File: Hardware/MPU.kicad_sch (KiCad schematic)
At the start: 18 parts, among them J6 USB_C_Receptacle_USB2.0_16P, U14 AP2112K-3.3, U2 STM32H723VGTx

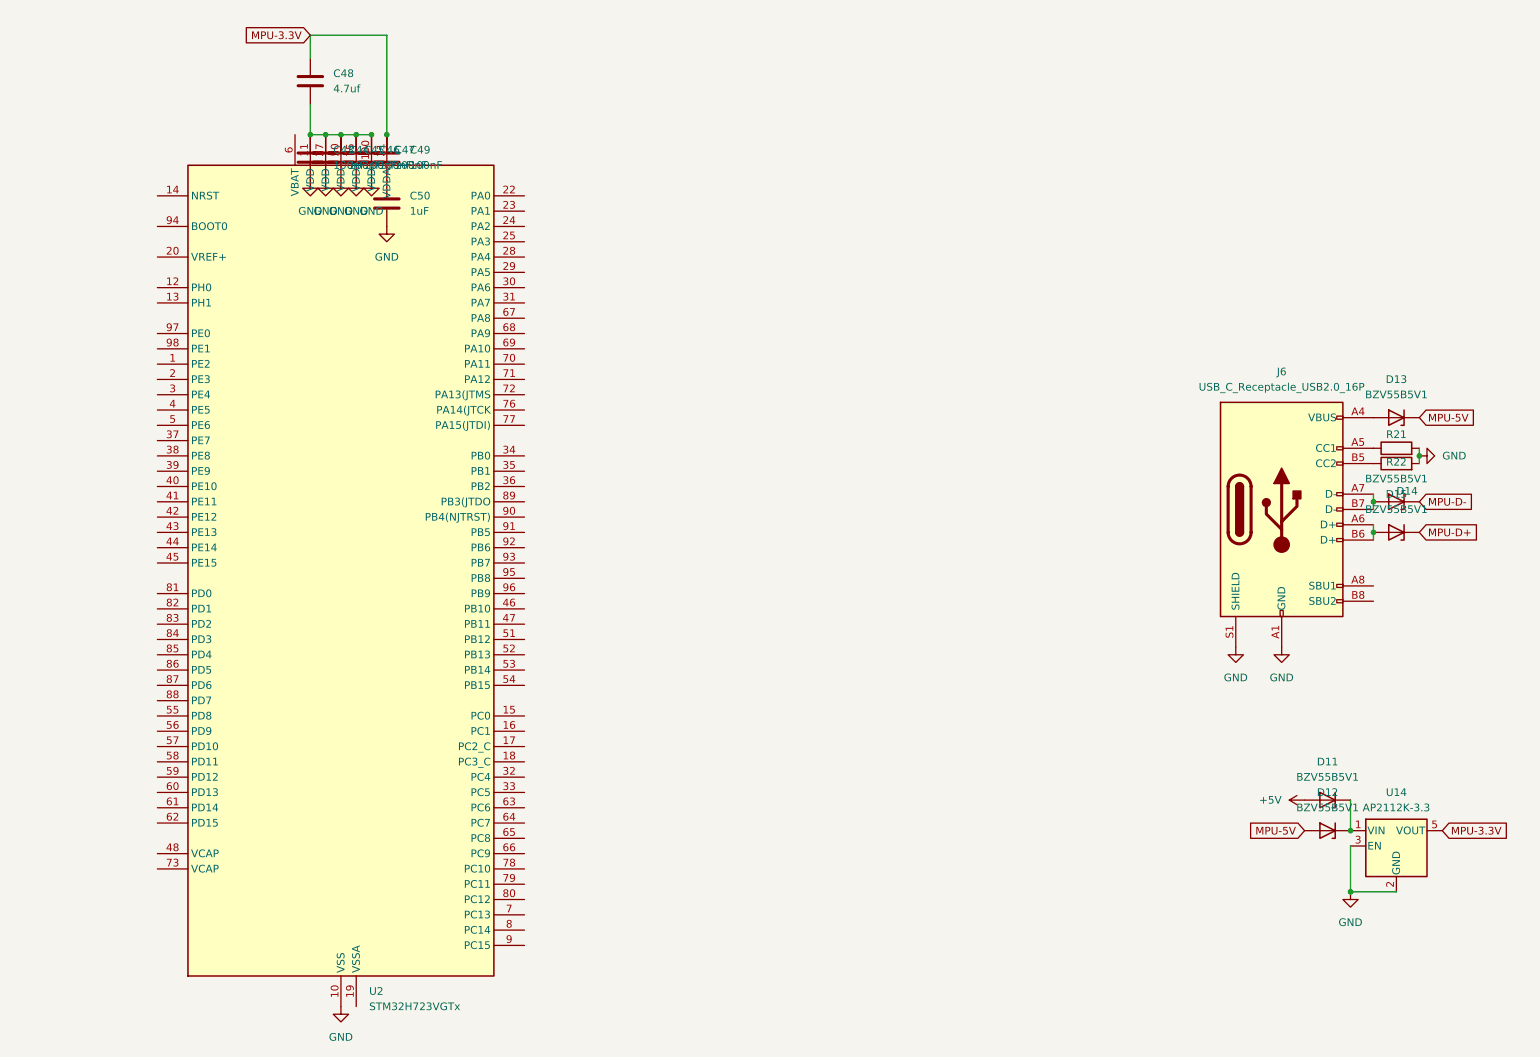
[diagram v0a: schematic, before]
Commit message: 19-feb update
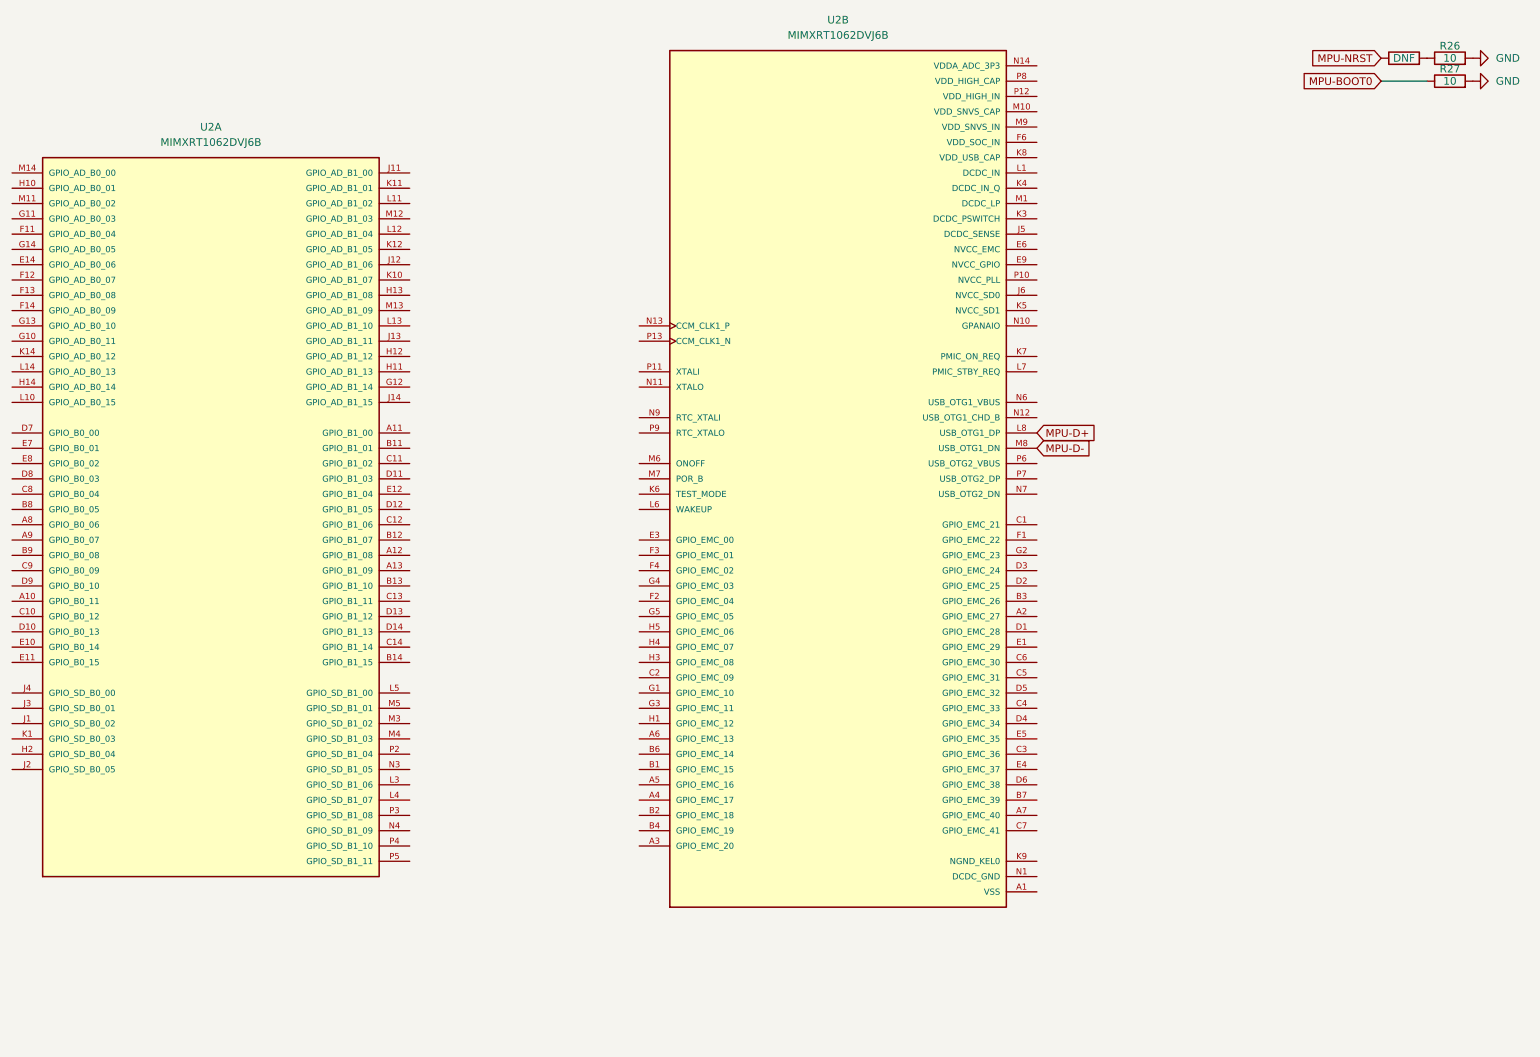
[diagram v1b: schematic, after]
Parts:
- removed C43, C44, C45, C46, C47, C49: 100nF, Capacitor_SMD:C_0201_0603Metric, symbol Device:C
- removed C48: 4.7uf, Capacitor_SMD:C_0603_1608Metric, symbol Device:C
- removed C50: 1uF, Capacitor_SMD:C_0201_0603Metric, symbol Device:C
- removed D11, D12, D13, D14, D15: BZV55B5V1, Diode_SMD:D_MiniMELF, symbol Diode:BZV55B5V1
- removed J6: USB_C_Receptacle_USB2.0_16P, Connector_USB:USB_C_Receptacle_G-Switch_GT-USB-7010ASV, symbol Connector:USB_C_Receptacle_USB2.0_16P
- removed R21, R22: R, Resistor_SMD:R_01005_0402Metric_Pad0.57x0.30mm_HandSolder, symbol Device:R
- removed U14: AP2112K-3.3, Package_TO_SOT_SMD:SOT-23-5, symbol Regulator_Linear:AP2112K-3.3
- removed U2: STM32H723VGTx, Package_QFP:LQFP-100_14x14mm_P0.5mm, symbol MCU_ST_STM32H7:STM32H723VGTx
- added R25: DNF, Resistor_SMD:R_0603_1608Metric, symbol Device:R
- added R26, R27: 10, Resistor_SMD:R_0201_0603Metric_Pad0.64x0.40mm_HandSolder, symbol Device:R
- added U2: MIMXRT1062DVJ6B, MIMXRT1062DVJ6B:BGA196C80P14X14_1200X1200X152N, symbol MIMXRT1062DVJ6B:MIMXRT1062DVJ6B
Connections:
- net GND: now also R26.2, R27.2
- net MPU-D+: now also U2.L8 (USB_OTG1_DP)
- net MPU-D-: now also U2.M8 (USB_OTG1_DN)
- new net: R25.2, R26.1
- new net DCDC_GND: U2.N1 (DCDC_GND), U2.N2 (DCDC_GND)
- new net DCDC_IN: U2.L1 (DCDC_IN), U2.L2 (DCDC_IN)
- new net DCDC_LP: U2.M1 (DCDC_LP), U2.M2 (DCDC_LP)
- new net MPU-BOOT0: R27.1
- new net MPU-NRST: R25.1
- new net NVCC_EMC: U2.E6 (NVCC_EMC), U2.F5 (NVCC_EMC)
- new net NVCC_GPIO: U2.E9 (NVCC_GPIO), U2.F10 (NVCC_GPIO), U2.J10 (NVCC_GPIO)
- new net VDD_SOC_IN: U2.F6 (VDD_SOC_IN), U2.F7 (VDD_SOC_IN), U2.F8 (VDD_SOC_IN), U2.F9 (VDD_SOC_IN), U2.G6 (VDD_SOC_IN), U2.G9 (VDD_SOC_IN), U2.H6 (VDD_SOC_IN), U2.H9 (VDD_SOC_IN), U2.J9 (VDD_SOC_IN)
- new net VSS: U2.A1 (VSS), U2.A14 (VSS), U2.B10 (VSS), U2.B5 (VSS), U2.E13 (VSS), U2.E2 (VSS), U2.G7 (VSS), U2.G8 (VSS), U2.H7 (VSS), U2.H8 (VSS), U2.J7 (VSS), U2.J8 (VSS), U2.K13 (VSS), U2.K2 (VSS), U2.L9 (VSS), U2.N5 (VSS), U2.N8 (VSS), U2.P1 (VSS), U2.P14 (VSS)
